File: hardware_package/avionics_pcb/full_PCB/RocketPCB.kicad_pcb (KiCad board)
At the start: 4 copper layers, 0.8 x 1 mm, 72 parts, among them J1 DX07S024XJ1R1100, J2 Micro_SD_Card, J3 Conn_01x03_Female, M1 Motor_Servo_JR, M2 Motor_Servo_JR, Q1 DMG2301L, Q2 DMG2301L, SW1 SW_Push, SW2 SW_Push, U1 STM32F405RGTx, U2 UCC381DP-3, U3 Radio_Header, U4 MPU6050_BO_FP, U5 W25Q16JV, U7 MPL3115A2, U8 GPS_header, U9 TPS63060

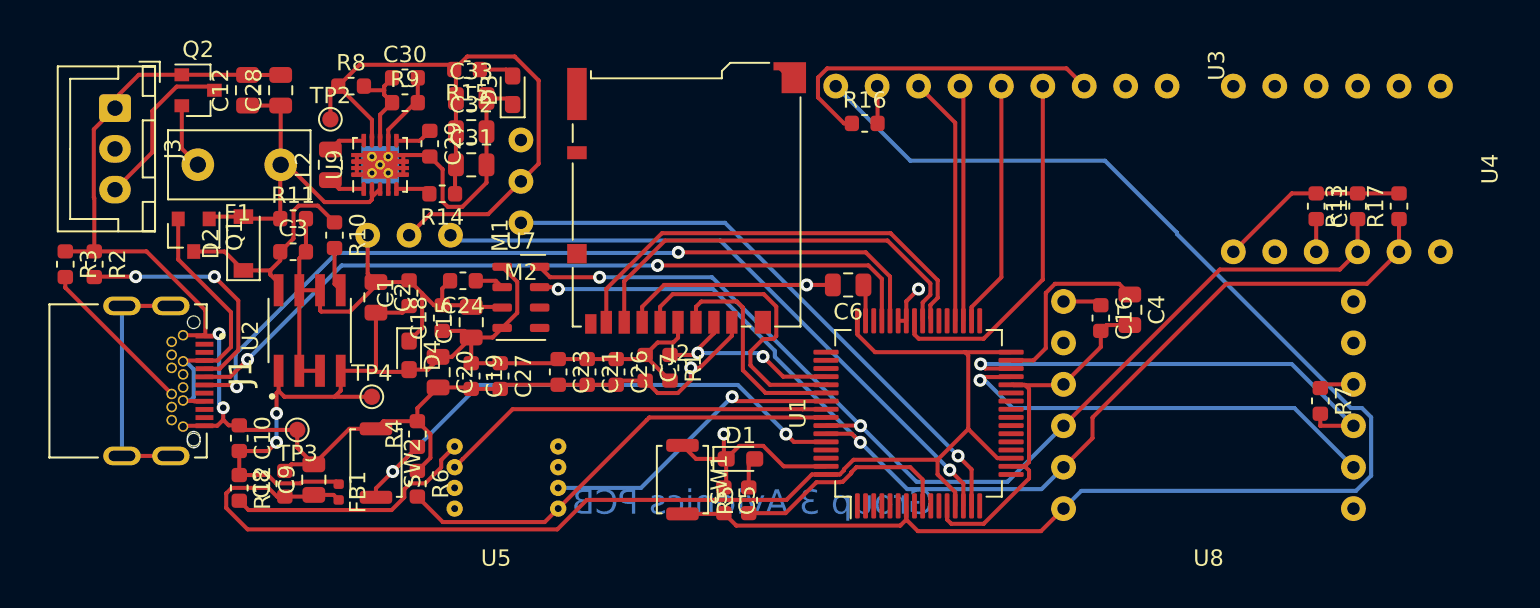
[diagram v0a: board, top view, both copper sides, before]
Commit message: Updated with the correct version
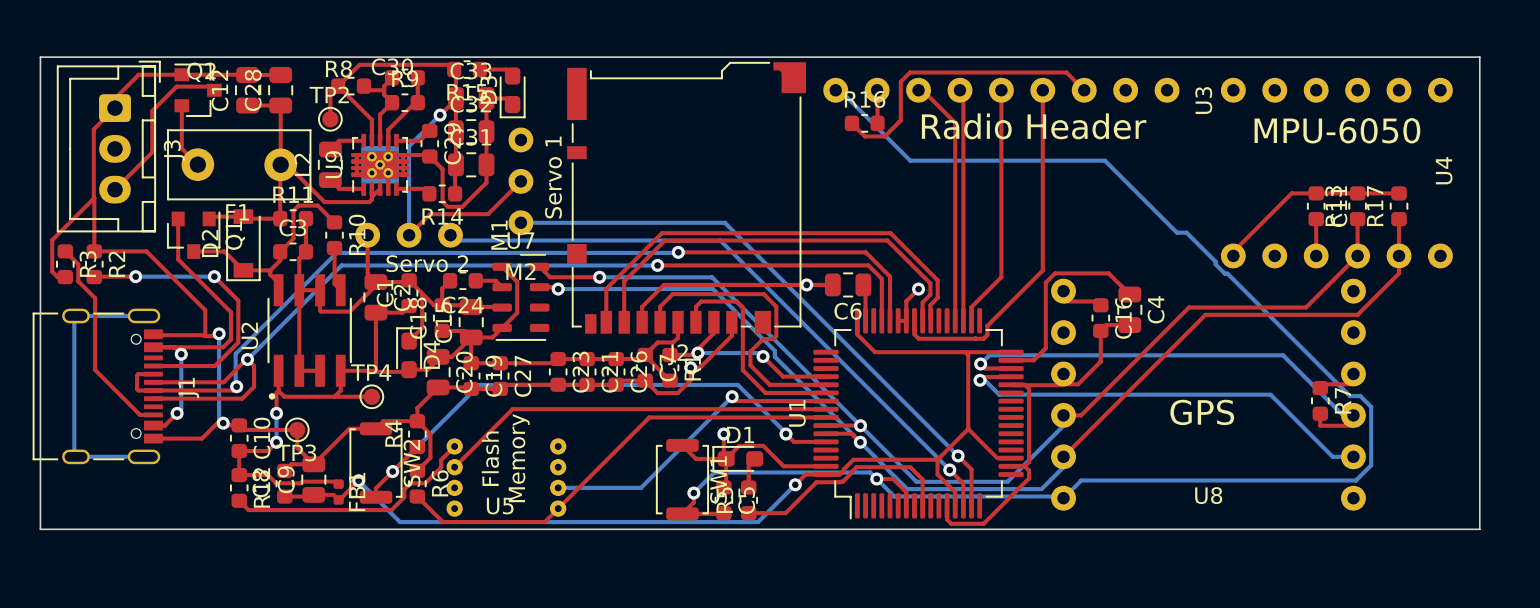
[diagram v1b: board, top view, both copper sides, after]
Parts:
- J1: value DX07S024XJ1R1100 -> USB_C_Receptacle; footprint DX07S024XJ1R1100:JAE_DX07S024XJ1R1100 -> Connector_USB:USB_C_Receptacle_Palconn_UTC16-G
- moved J1 6.35 mm to (69.4, 75.6)
- moved U8 0.64 mm to (136.7, 83.7)
- moved U3 0.25 mm to (135.4, 57.4)
- moved U4 0.25 mm to (153.4, 62.5)
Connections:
- R3 pad 1: GND -> Net-(J1-PadB5)
- R3 pad 2: Net-(J1-PadB5) -> GND
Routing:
- net /D+: track 47.3 -> 59.1 mm
- net Net-(C8-Pad1): track 79.1 -> 68.2 mm, vias 0 -> 2
- net GND: track 201.3 -> 211.2 mm
- net /D-: track 50.1 -> 56.1 mm
- net ~RESET~: track 90.1 -> 95.3 mm, vias 0 -> 2
- net VBUS: track 17.1 -> 21.2 mm, vias 0 -> 2
- net +6V: track 43.0 -> 39.8 mm, vias 0 -> 1
- net +3V3: track 114.2 -> 111.3 mm
- net Net-(J1-PadA5): track 15.0 -> 17.9 mm
- net Net-(J1-PadB5): track 9.87 -> 12.7 mm
- net Net-(J1-PadS1): track 15.2 -> 17.0 mm
- net Net-(C4-Pad1): track 11.5 -> 12.4 mm
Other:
- board size 0.8 x 1 mm -> 88.3 x 29 mm
- board text added: "Avionics Package - Project Beans"
- board text added: "Flash Memory"
- board text added: "GPS"
- board text added: "MPU-6050"
- board text added: "Radio Header"
- board text added: "Servo 1"
- board text added: "Servo 2"
- board text removed: "Group 3 Avionics PCB"
